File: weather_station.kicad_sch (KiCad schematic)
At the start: 0 parts

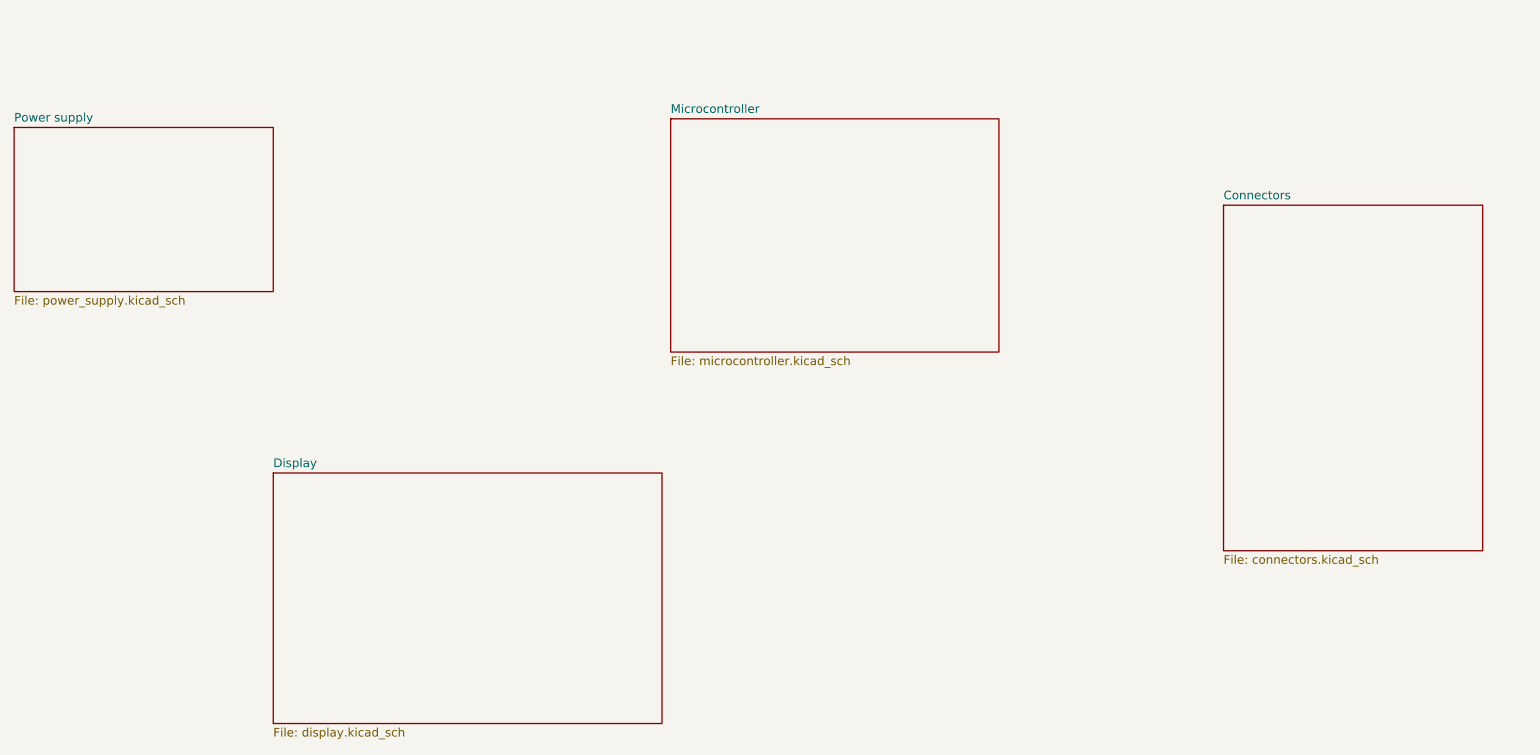
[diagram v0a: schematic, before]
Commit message: Finished schematic and first layout
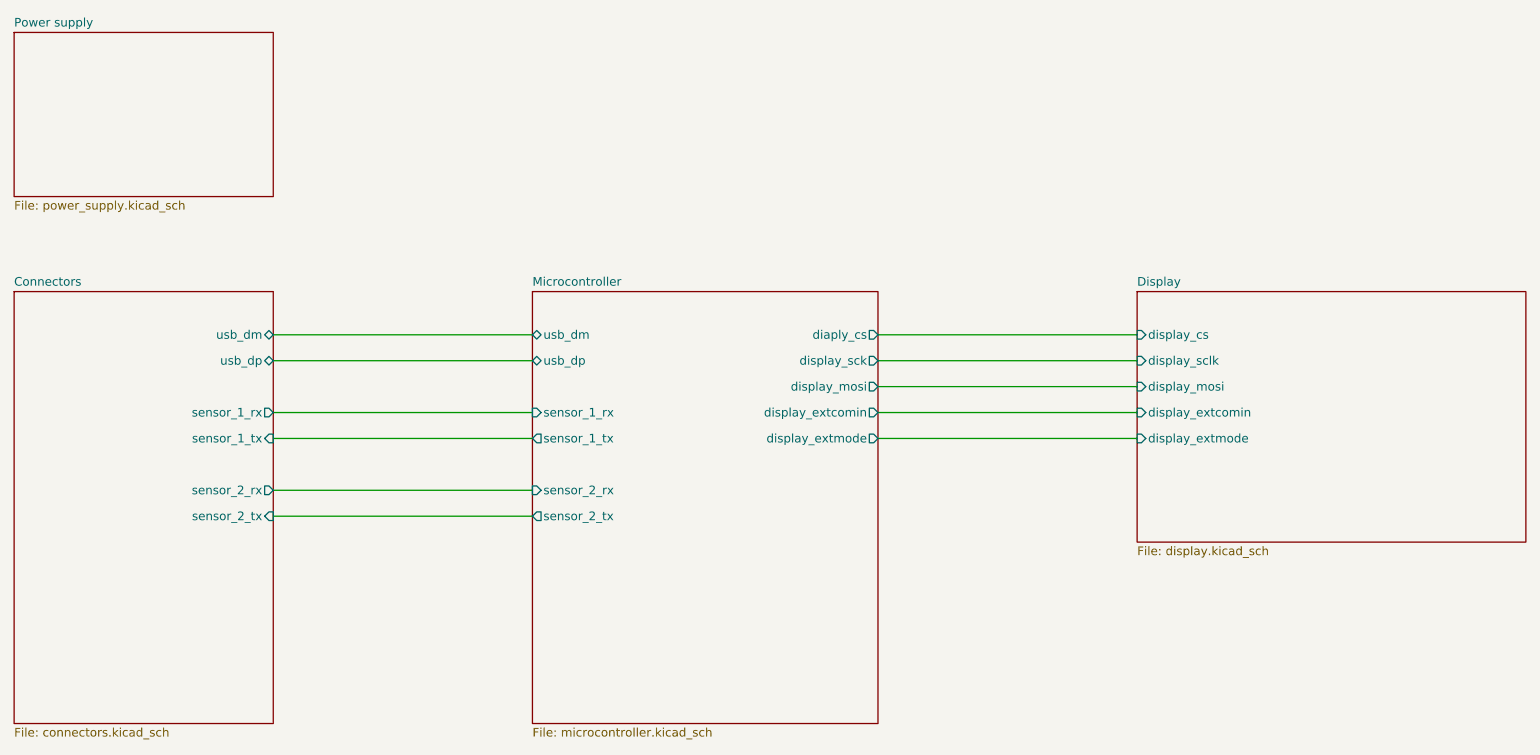
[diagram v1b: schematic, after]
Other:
- sheet Connectors ports: added sensor_1_rx, sensor_1_tx, sensor_2_rx, sensor_2_tx, usb_dm, usb_dp; removed none
- sheet Display ports: added display_cs, display_extcomin, display_extmode, display_mosi, display_sclk; removed none
- sheet Microcontroller ports: added diaply_cs, display_extcomin, display_extmode, display_mosi, display_sck, sensor_1_rx, sensor_1_tx, sensor_2_rx, sensor_2_tx, usb_dm, usb_dp; removed none
